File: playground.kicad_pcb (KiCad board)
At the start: 2 copper layers, 72 x 68 mm, 70 parts, among them IC1 TXU0101DBVR, IC11 LM3940IMP-3.3_NOPB, IC2 TXU0101DBVR, IC3 TXU0101DBVR, IC4 TXU0101DBVR, IC5 TXU0101DBVR, IC6 TXU0101DBVR, IC7 TXU0101DBVR, IC8 TXU0101DBVR, IC9 L293DD, J1 67643-2910, J2 Pump, J3 Fan, J4 Valve, J5 Conn_02x05_Counter_Clockwise, J6 MOLEX POWER CONNECTOR, SW1 SW_DIP_x01, U2 ATSAMD21G18A-A, Y1 32.768kHz

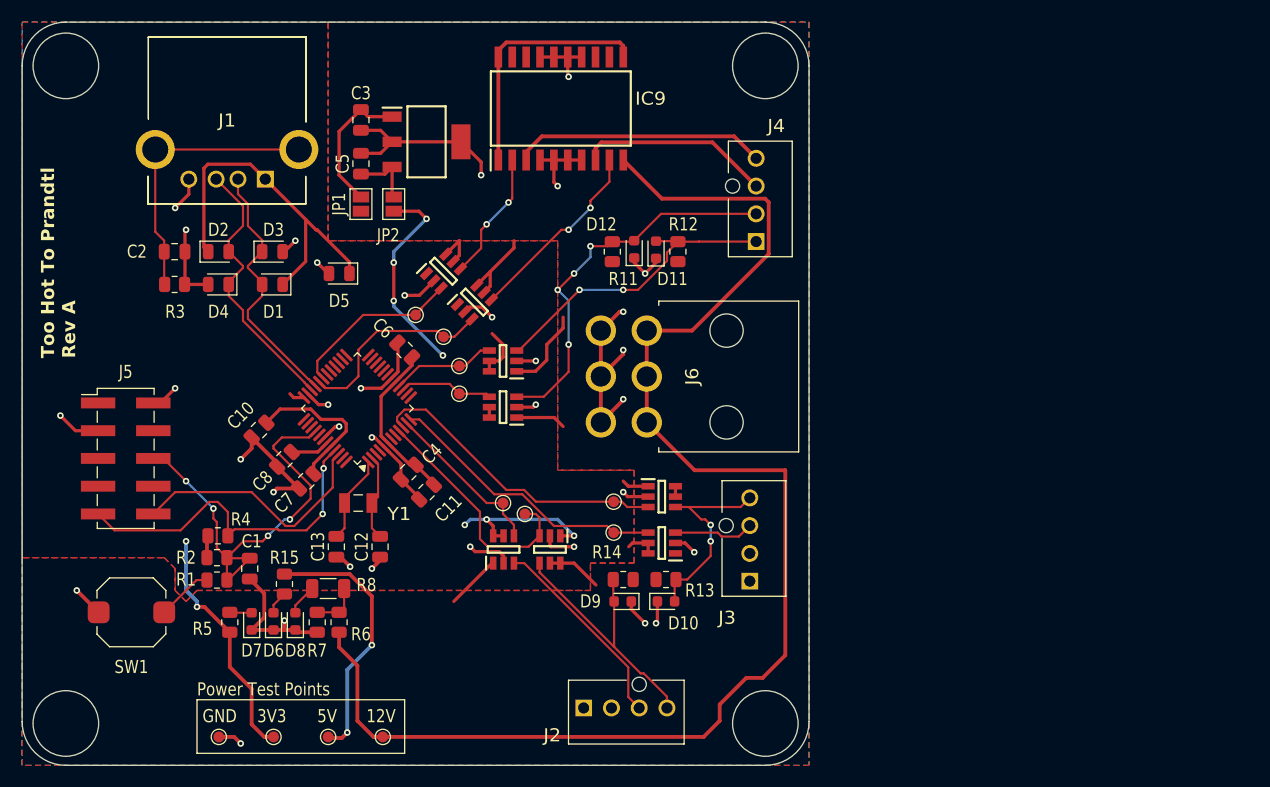
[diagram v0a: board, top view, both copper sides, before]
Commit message: Initial Layout
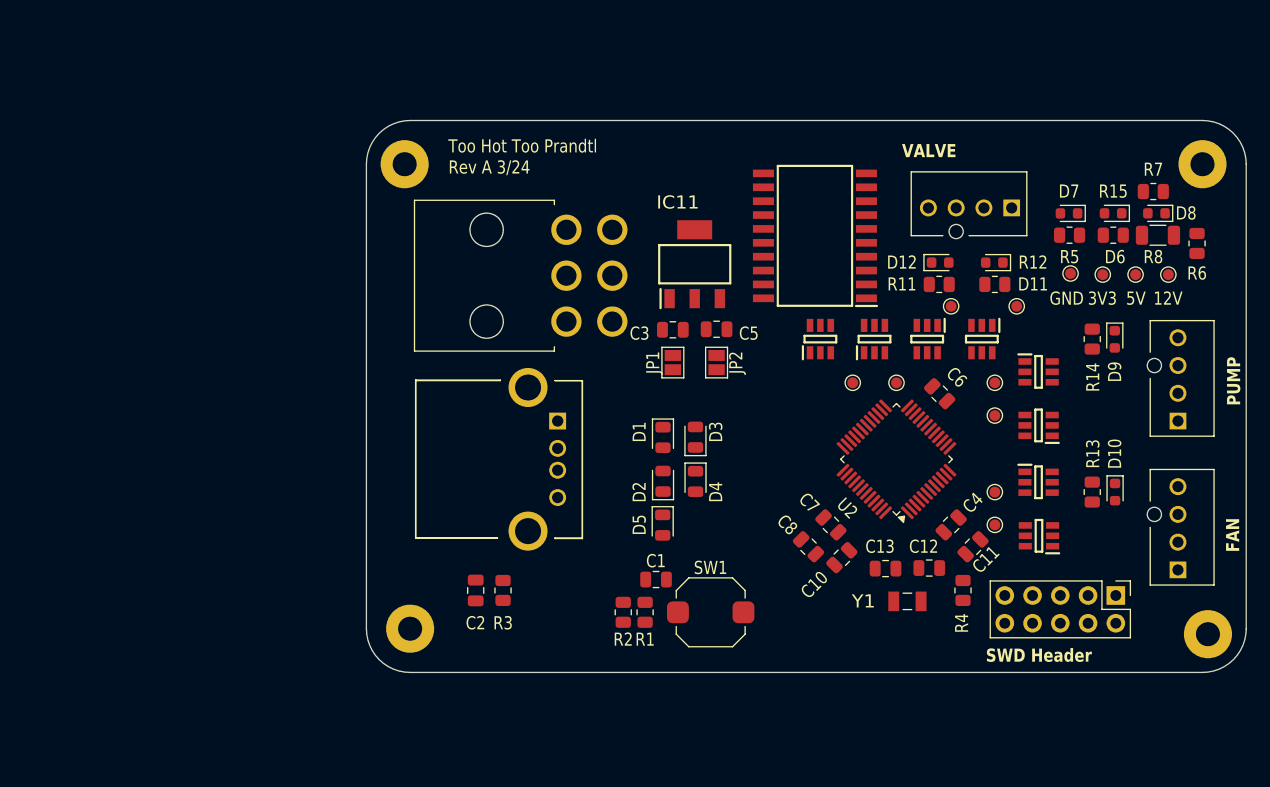
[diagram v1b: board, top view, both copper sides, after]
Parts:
- added H1: MountingHole_Pad, MountingHole:MountingHole_2.2mm_M2_Pad, F.Cu at (158.0, 63.0)
- added H2: MountingHole_Pad, MountingHole:MountingHole_2.2mm_M2_Pad, F.Cu at (158.5, 106.0)
- added H3: MountingHole_Pad, MountingHole:MountingHole_2.2mm_M2_Pad, F.Cu at (85.0, 63.0)
- added H4: MountingHole_Pad, MountingHole:MountingHole_2.2mm_M2_Pad, F.Cu at (85.5, 105.5)
- J5: footprint Connector_PinHeader_2.54mm:PinHeader_2x05_P2.54mm_Vertical_SMD -> Connector_PinHeader_2.54mm:PinHeader_2x05_P2.54mm_Vertical
- moved J5 91.5 mm to (150.1, 102.5), turned to -90 degrees
- moved TP4 88.7 mm to (145.9, 73.0)
- moved D8 87.2 mm to (153.8, 67.5), turned to 180 degrees
- moved TP3 86.9 mm to (148.9, 73.1)
- moved R7 86.1 mm to (153.5, 65.5), turned to 0 degrees
- moved R6 85.8 mm to (157.5, 70.2)
- moved D6 85.4 mm to (149.8, 67.5), turned to 180 degrees
- moved TP2 85.1 mm to (151.9, 73.1)
- moved R5 84.6 mm to (145.8, 69.5), turned to 0 degrees
- moved D7 83.6 mm to (145.8, 67.5), turned to 180 degrees
- moved TP1 83.4 mm to (154.9, 73.1)
- moved R8 82.5 mm to (153.9, 69.5)
- moved R15 82.3 mm to (149.8, 69.5), turned to 0 degrees
- moved R4 68.4 mm to (136.1, 102.0), turned to -90 degrees
- moved J2 60.4 mm to (155.8, 86.5), turned to -90 degrees
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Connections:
- net Net-(R1-Pad1) renamed /RST_SW_R
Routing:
- net GND: track 146.4 -> 0.00 mm, vias 34 -> 0
- net +12V: track 126.0 -> 0.00 mm
- net +5V: track 114.8 -> 0.00 mm, vias 2 -> 0
- net +3V3: track 103.4 -> 0.00 mm, vias 9 -> 0
- net /RESET: track 40.0 -> 0.00 mm, vias 4 -> 0
- net /ValveSense1_5v: track 35.2 -> 0.00 mm, vias 4 -> 0
- net /SWCLK: track 32.0 -> 0.00 mm, vias 2 -> 0
- net /ValveSense2_5v: track 28.5 -> 0.00 mm, vias 2 -> 0
- net /FanCtrl_3v3: track 28.1 -> 0.00 mm
- net /FanSense_3v3: track 26.0 -> 0.00 mm
- net /usb_shield_gnd: track 25.8 -> 0.00 mm
- net /USB_D+: track 25.1 -> 0.00 mm
- net /PumpCtrl_5v: track 24.4 -> 0.00 mm
- net /USB_D-: track 24.1 -> 0.00 mm
- net /SWDIO: track 23.3 -> 0.00 mm
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- removed copper zone on F.Cu, net +3V3
- removed copper zone on F.Cu, net +5V
- removed copper zone on B.Cu, net GND
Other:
- board size 72 x 68 mm -> 80.5 x 50.5 mm
- copper layers 2 -> 4
- board text added: "FAN"
- board text added: "PUMP"
- board text added: "SWD Header"
- board text added: "Too Hot Too Prandtl Rev A 3/24"
- board text added: "VALVE"
- board text removed: "Power Test Points"
- board text removed: "Too Hot To Prandtl Rev A"
